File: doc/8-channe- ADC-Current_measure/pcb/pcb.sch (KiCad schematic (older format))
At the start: 31 parts

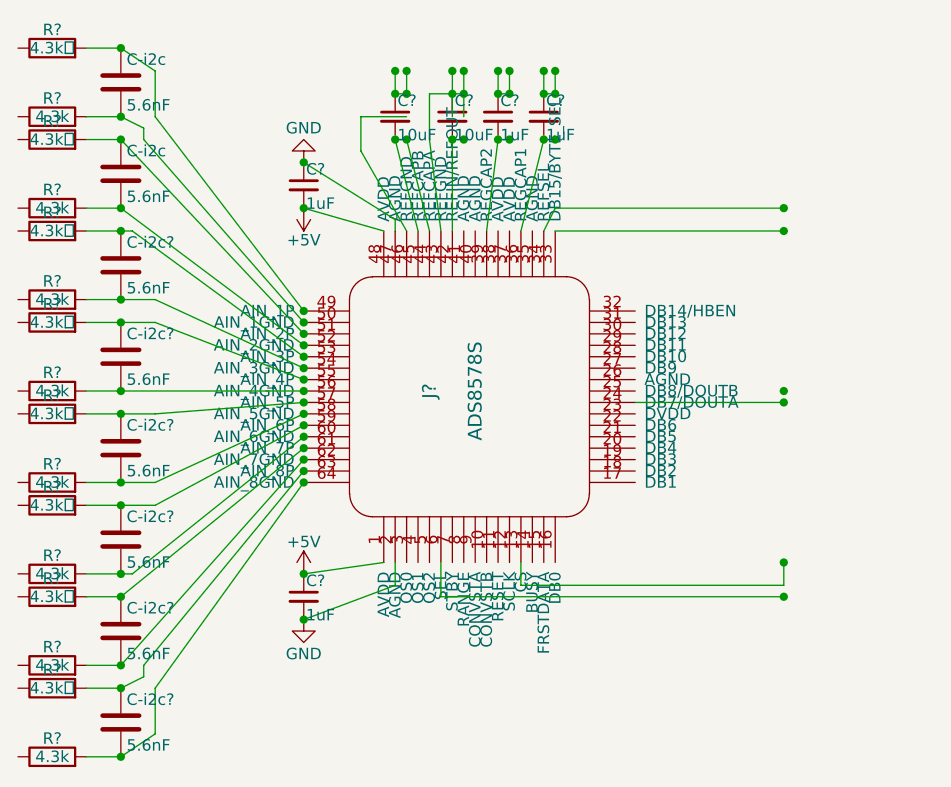
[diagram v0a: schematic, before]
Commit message: semi-ready
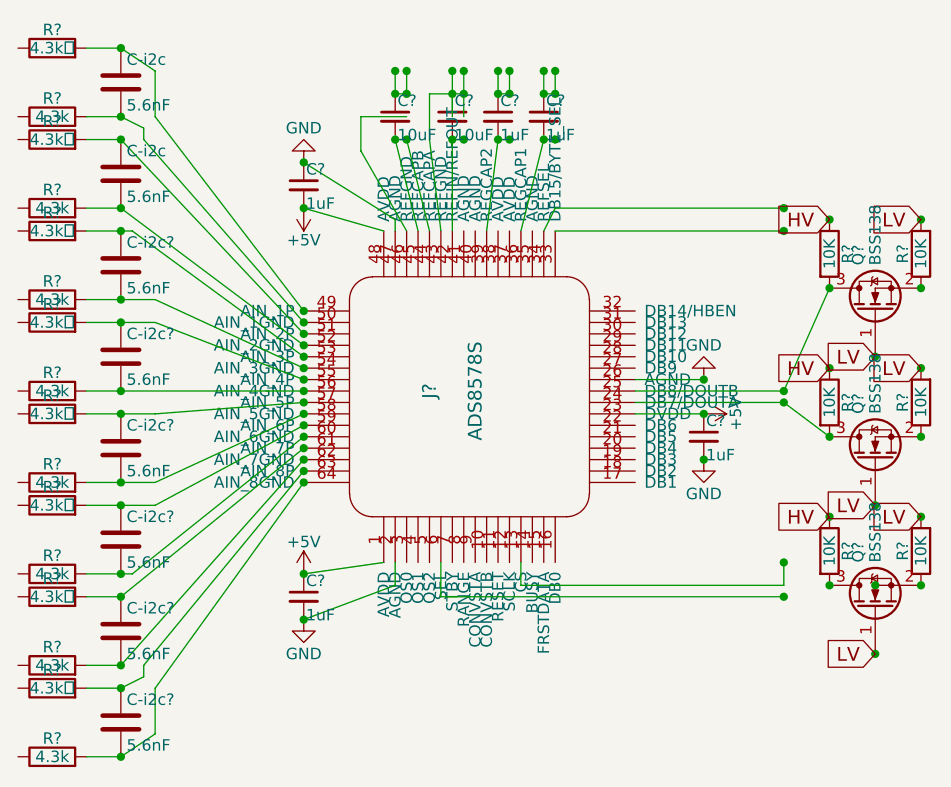
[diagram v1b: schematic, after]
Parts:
- added C?: 1uF, symbol C_Small
- added Q? (x3): BSS138, TO_SOT_Packages_SMD:SOT-23, symbol BSS138
- added R? (x6): 10K, symbol R
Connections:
- net labels added: HV, LV
- wire segments 80 -> 85
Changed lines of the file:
@@
 	5650 4750 7150 4750
 Connection ~ 7150 4750
+Wire Wire Line
+	6500 3850 7150 3850
+$Comp
+L BSS138 Q?
+U 1 1 5A924864
+P 7550 4150
+F 0 "Q?" H 7750 4225 50  0000 L CNN
+F 1 "BSS138" H 7750 4150 50  0000 L CNN
+F 2 "TO_SOT_Packages_SMD:SOT-23" H 7750 4075 50  0001 L CIN
+F 3 "" H 7550 4150 50  0001 L CNN
+	1    7550 4150
+	0    -1   -1   0
+$EndComp
+$Comp
+L BSS138 Q?
+U 1 1 5A924979
+P 7550 4800
+F 0 "Q?" H 7750 4875 50  0000 L CNN
+F 1 "BSS138" H 7750 4800 50  0000 L CNN
+F 2 "TO_SOT_Packages_SMD:SOT-23" H 7750 4725 50  0001 L CIN
+F 3 "" H 7550 4800 50  0001 L CNN
+	1    7550 4800
+	0    -1   -1   0
+$EndComp
+$Comp
+L BSS138 Q?
+U 1 1 5A924C5C
+P 7550 3500
+F 0 "Q?" H 7750 3575 50  0000 L CNN
+F 1 "BSS138" H 7750 3500 50  0000 L CNN
+F 2 "TO_SOT_Packages_SMD:SOT-23" H 7750 3425 50  0001 L CIN
+F 3 "" H 7550 3500 50  0001 L CNN
+	1    7550 3500
+	0    -1   -1   0
+$EndComp
+Wire Wire Line
+	7150 3850 7350 3400
+Connection ~ 7350 3400
+Connection ~ 7350 4050
+Connection ~ 7350 4700
+Connection ~ 7750 4700
+Connection ~ 7750 4050
+Connection ~ 7750 3400
+Connection ~ 7550 4700
+$Comp
+L R R?
+U 1 1 5A9255F8
+P 7750 3250
+F 0 "R?" V 7830 3250 50  0000 C CNN
+F 1 "10K" V 7750 3250 50  0000 C CNN
+F 2 "" V 7680 3250 50  0001 C CNN
+F 3 "" H 7750 3250 50  0001 C CNN
+	1    7750 3250
+	-1   0    0    1
+$EndComp
+Wire Wire Line
+	7150 3900 7350 4050
+$Comp
+L R R?
+U 1 1 5A9261F2
+P 7750 3900
+F 0 "R?" V 7830 3900 50  0000 C CNN
+F 1 "10K" V 7750 3900 50  0000 C CNN
+F 2 "" V 7680 3900 50  0001 C CNN
+F 3 "" H 7750 3900 50  0001 C CNN
+	1    7750 3900
+	-1   0    0    1
+$EndComp
+$Comp
+L R R?
+U 1 1 5A926286
+P 7750 4550
+F 0 "R?" V 7830 4550 50  0000 C CNN
+F 1 "10K" V 7750 4550 50  0000 C CNN
+F 2 "" V 7680 4550 50  0001 C CNN
+F 3 "" H 7750 4550 50  0001 C CNN
+	1    7750 4550
+	-1   0    0    1
+$EndComp
+Connection ~ 7750 4400
+Connection ~ 7750 3750
+Connection ~ 7750 3100
+$Comp
+L R R?
+U 1 1 5A926302
+P 7350 3900
+F 0 "R?" V 7430 3900 50  0000 C CNN
+F 1 "10K" V 7350 3900 50  0000 C CNN
+F 2 "" V 7280 3900 50  0001 C CNN
+F 3 "" H 7350 3900 50  0001 C CNN
+	1    7350 3900
+	1    0    0    -1
+$EndComp
+$Comp
+L R R?
+U 1 1 5A926375
+P 7350 3250
+F 0 "R?" V 7430 3250 50  0000 C CNN
+F 1 "10K" V 7350 3250 50  0000 C CNN
+F 2 "" V 7280 3250 50  0001 C CNN
+F 3 "" H 7350 3250 50  0001 C CNN
+	1    7350 3250
+	1    0    0    -1
+$EndComp
+$Comp
+L R R?
+U 1 1 5A926422
+P 7350 4550
+F 0 "R?" V 7430 4550 50  0000 C CNN
+F 1 "10K" V 7350 4550 50  0000 C CNN
+F 2 "" V 7280 4550 50  0001 C CNN
+F 3 "" H 7350 4550 50  0001 C CNN
+	1    7350 4550
+	1    0    0    -1
+$EndComp
+Connection ~ 7350 3750
+Connection ~ 7350 3100
+Connection ~ 7350 4400
+Connection ~ 7550 5000
+Connection ~ 7550 4350
+Connection ~ 7550 3700
+Text GLabel 7550 5000 0    60   Input ~ 0
+LV
+Text GLabel 7550 4350 0    60   Input ~ 0
+LV
+Text GLabel 7550 3700 0    60   Input ~ 0
+LV
+Text GLabel 7750 3100 0    60   Input ~ 0
+LV
+Text GLabel 7750 3750 0    60   Input ~ 0
+LV
+Text GLabel 7750 4400 0    60   Input ~ 0
+LV
+Text GLabel 7350 3100 0    60   Input ~ 0
+HV
+Text GLabel 7350 3750 0    60   Input ~ 0
+HV
+Text GLabel 7350 4400 0    60   Input ~ 0
+HV
+Wire Wire Line
+	6500 3950 6800 3950
+Wire Wire Line
+	6500 3800 6800 3800
+$Comp
+L GND #PWR?
+U 1 1 5A926E97
+P 6800 3800
+F 0 "#PWR?" H 6800 3550 50  0001 C CNN
+F 1 "GND" H 6800 3650 50  0000 C CNN
+F 2 "" H 6800 3800 50  0001 C CNN
+F 3 "" H 6800 3800 50  0001 C CNN
+	1    6800 3800
+	-1   0    0    1
+$EndComp
+$Comp
+L +5V #PWR?
+U 1 1 5A926F1A
+P 6800 3950
+F 0 "#PWR?" H 6800 3800 50  0001 C CNN
+F 1 "+5V" H 6800 4090 50  0000 C CNN
+F 2 "" H 6800 3950 50  0001 C CNN
+F 3 "" H 6800 3950 50  0001 C CNN
+	1    6800 3950
+	0    1    1    0
+$EndComp
+Connection ~ 6800 3950
+Connection ~ 6800 3800
+$Comp
+L C_Small C?
+U 1 1 5A9271A4
+P 6800 4050
+F 0 "C?" H 6810 4120 50  0000 L CNN
+F 1 "1uF" H 6810 3970 50  0000 L CNN
+F 2 "" H 6800 4050 50  0001 C CNN
+F 3 "" H 6800 4050 50  0001 C CNN
+	1    6800 4050
+	1    0    0    -1
+$EndComp
+$Comp
+L GND #PWR?
+U 1 1 5A927269
+P 6800 4150
+F 0 "#PWR?" H 6800 3900 50  0001 C CNN
+F 1 "GND" H 6800 4000 50  0000 C CNN
+F 2 "" H 6800 4150 50  0001 C CNN
+F 3 "" H 6800 4150 50  0001 C CNN
+	1    6800 4150
+	1    0    0    -1
+$EndComp
+Connection ~ 6800 4150
 $EndSCHEMATC
